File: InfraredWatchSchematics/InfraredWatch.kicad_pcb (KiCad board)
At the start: 4 copper layers, 84.1 x 40.3 mm, 51 parts, among them J2 Micro_SD_Card_Det2, J4 USB_C_Receptacle_USB2.0_16P, P1 XC9265A331MR-G, U1 MCP73831-5-OT, U2 USBLC6-2SC6, U3 STM32WB55CGU6, U4 A1001312, Y1 32.768kHz, Y2 32MHz

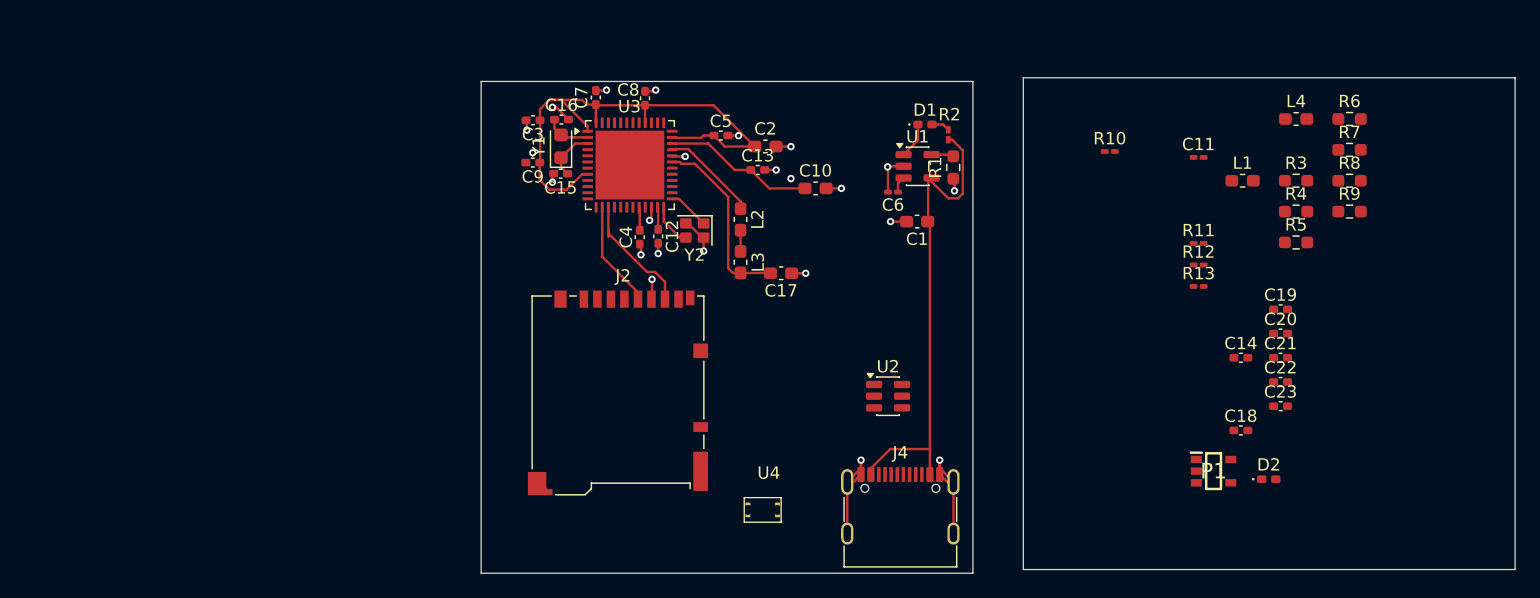
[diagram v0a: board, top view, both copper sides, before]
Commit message: Wed Apr 29 09:42:28 EDT 2026 | updated pcb
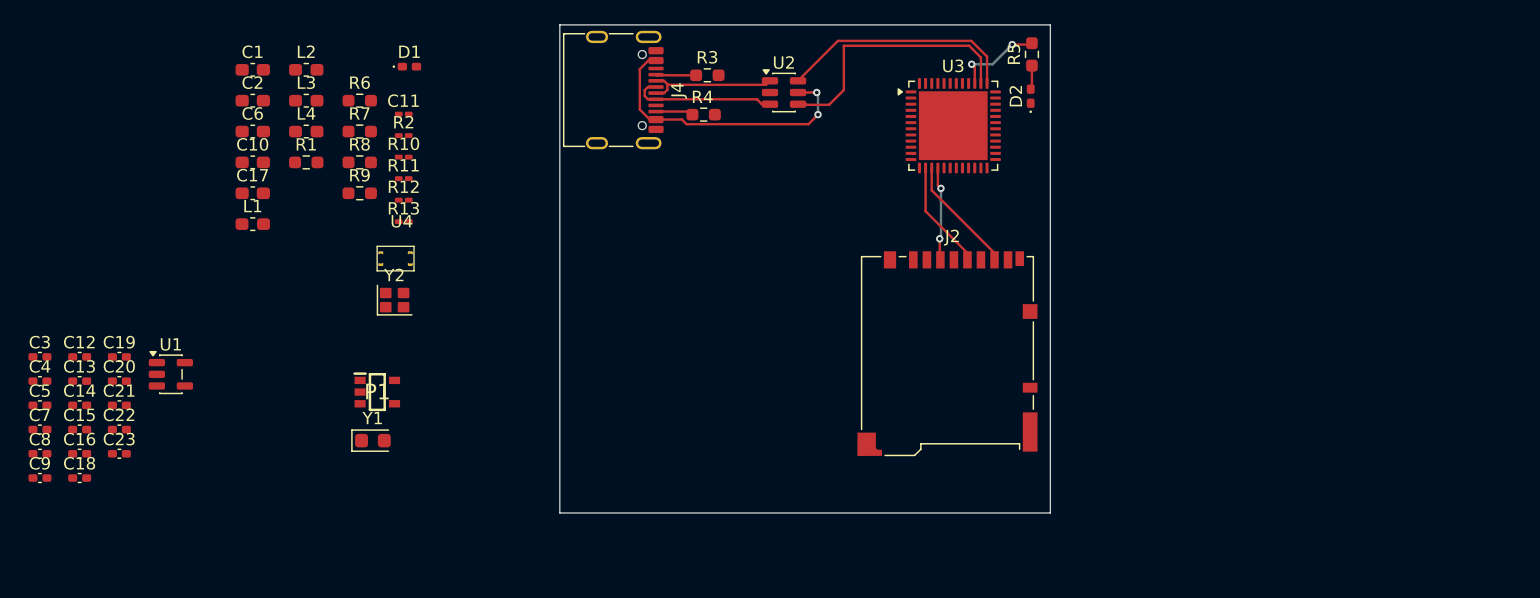
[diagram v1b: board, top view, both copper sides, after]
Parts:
- C6: footprint Capacitor_SMD:C_0201_0603Metric_Pad0.64x0.40mm_HandSolder -> Capacitor_SMD:C_0603_1608Metric_Pad1.08x0.95mm_HandSolder
- moved C19 94.5 mm to (94.5, 115.7)
- moved C20 94.5 mm to (94.5, 117.7)
- moved C21 94.5 mm to (94.5, 119.6)
- moved C22 94.5 mm to (94.5, 121.6)
- moved C23 94.5 mm to (94.5, 123.6)
- moved C14 94.5 mm to (91.2, 119.6)
- moved C18 94.5 mm to (91.2, 125.6)
- moved L1 80.6 mm to (105.3, 104.9)
- moved R6 80.5 mm to (114.0, 94.9)
- moved R7 80.5 mm to (114.0, 97.4)
- moved R8 80.5 mm to (114.0, 99.9)
- moved R9 80.5 mm to (114.0, 102.4)
- moved L4 80.5 mm to (109.7, 97.4)
- moved P1 68.3 mm to (115.5, 118.6)
- moved R11 64.9 mm to (117.6, 101.2)
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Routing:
- net Power: track 60.9 -> 0.00 mm
- net GND: track 42.2 -> 0.00 mm, vias 23 -> 0
- net /USB_D+: track 0.00 -> 22.2 mm
- net /USB_D-: track 0.00 -> 19.4 mm
- net CHARGE_IN: track 38.8 -> 23.6 mm, vias 0 -> 2
- net /SMBSFB: track 15.1 -> 0.00 mm
- net Net-(J4-D+-PadA6): track 0.00 -> 12.3 mm
- net Net-(J4-D--PadA7): track 0.00 -> 11.0 mm
- net /SMBSLX: track 7.94 -> 0.00 mm
- net /SD_MOSI: track 0.00 -> 7.64 mm, vias 0 -> 2
- net /IR: track 0.00 -> 7.28 mm, vias 0 -> 2
- net /LSE_Out: track 4.16 -> 0.00 mm
- net /LSE_In: track 3.72 -> 0.00 mm
- net /HSC_Out: track 3.49 -> 0.00 mm
- net /HSC_In: track 3.39 -> 0.00 mm
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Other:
- board size 84.1 x 40.3 mm -> 39.9 x 39.7 mm
